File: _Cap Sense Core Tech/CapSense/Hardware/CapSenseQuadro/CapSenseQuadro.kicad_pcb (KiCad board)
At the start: 2 copper layers, 30 x 51.3 mm, 48 parts, among them IC1 FDC2214-rescue_FDC2214QRGHRQ1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, IC2 FDC2214QRGHRQ1, J1 Conn_02x04_Odd_Even, J2 Conn_02x04_Odd_Even, J3 Conn_02x01, SW1 SW_Push_DPDT, Y1 ECS-2033-400-BN

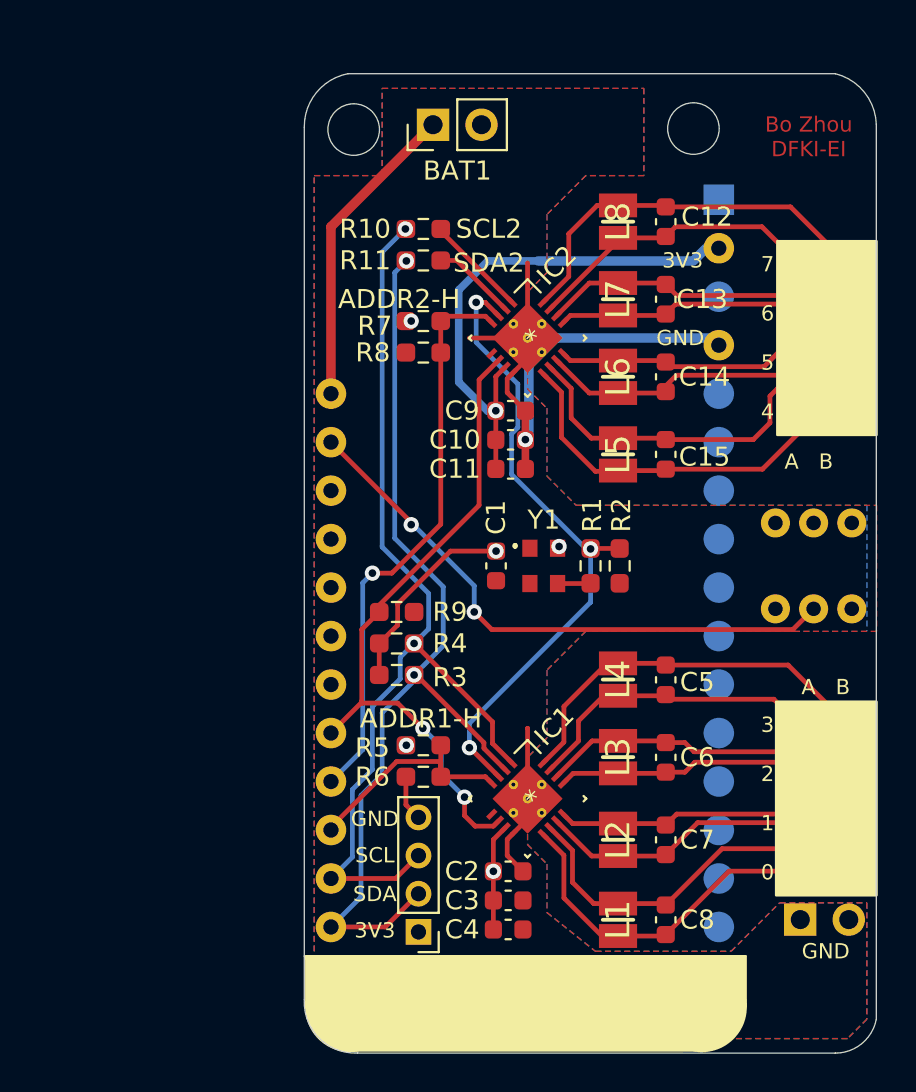
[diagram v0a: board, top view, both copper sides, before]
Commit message: pcb
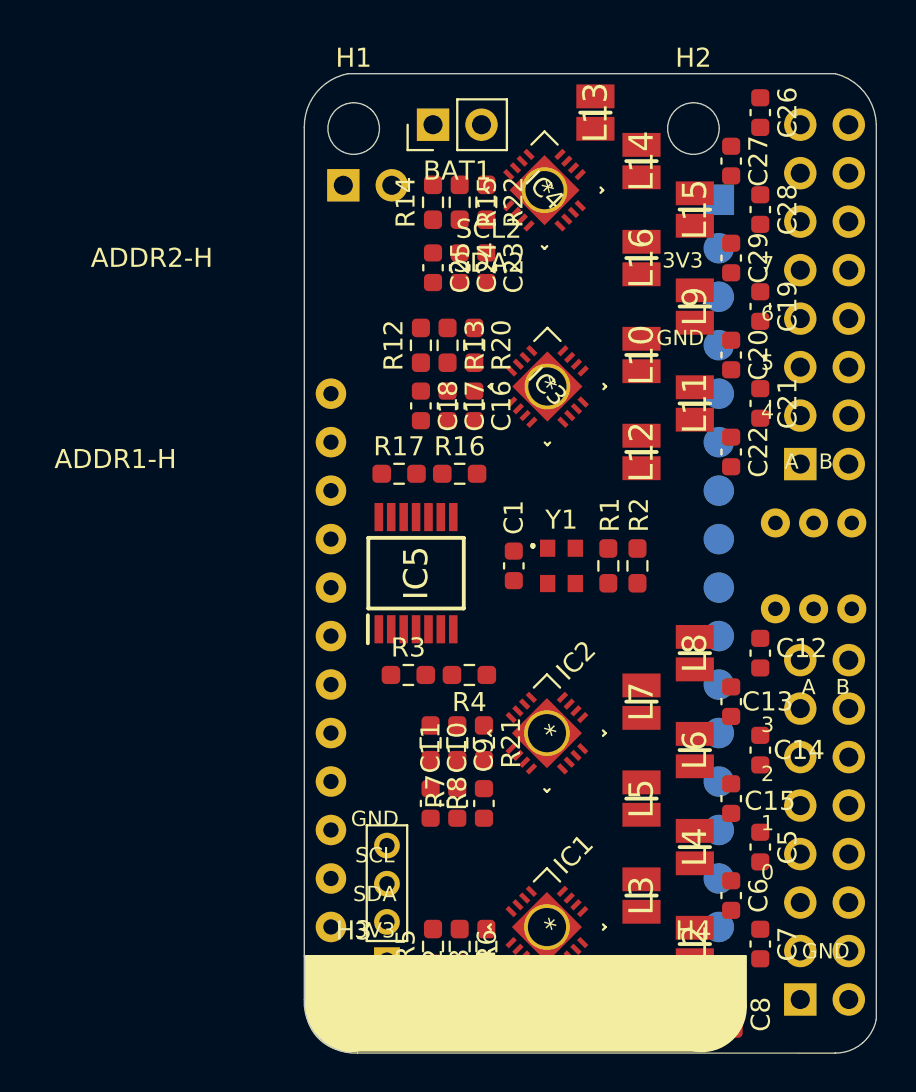
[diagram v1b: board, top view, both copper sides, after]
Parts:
- removed R10, R11: R, Resistor_SMD:R_0603_1608Metric_Pad0.98x0.95mm_HandSolder
- added C16: C, Capacitor_SMD:C_0603_1608Metric, F.Cu at (109.0, 117.2)
- added C17: C, Capacitor_SMD:C_0603_1608Metric, F.Cu at (107.6, 117.2)
- added C18: C, Capacitor_SMD:C_0603_1608Metric, F.Cu at (106.2, 117.2)
- added C19: Device_C, Capacitor_SMD:C_0603_1608Metric, F.Cu at (124.0, 112.0)
- added C20: Device_C, Capacitor_SMD:C_0603_1608Metric, F.Cu at (122.4, 114.6)
- added C21: Device_C, Capacitor_SMD:C_0603_1608Metric, F.Cu at (124.0, 117.1)
- added C22: Device_C, Capacitor_SMD:C_0603_1608Metric, F.Cu at (122.4, 119.6)
- added C23: C, Capacitor_SMD:C_0603_1608Metric, F.Cu at (109.6, 110.0)
- added C24: C, Capacitor_SMD:C_0603_1608Metric, F.Cu at (108.2, 110.0)
- added C25: C, Capacitor_SMD:C_0603_1608Metric, F.Cu at (106.8, 110.0)
- added C26: Device_C, Capacitor_SMD:C_0603_1608Metric, F.Cu at (124.0, 101.9)
- added C27: Device_C, Capacitor_SMD:C_0603_1608Metric, F.Cu at (122.4, 104.4)
- added C28: Device_C, Capacitor_SMD:C_0603_1608Metric, F.Cu at (124.0, 106.9)
- added C29: Device_C, Capacitor_SMD:C_0603_1608Metric, F.Cu at (122.4, 109.5)
- added IC3: FDC2214QRGHRQ1, FDC2214:FDC2214RGHR, F.Cu at (112.8, 116.2)
- added IC4: FDC2214QRGHRQ1, FDC2214:FDC2214RGHR, F.Cu at (112.6, 105.9)
- added IC5: PCA9543APWR, SamacSys:SOP65P640X120-14N, F.Cu at (105.9, 126.0)
- added L10: L0806C470MPWST, SamacSys:INDC2018X180N, F.Cu at (117.7, 114.6)
- added L11: L0806C470MPWST, SamacSys:INDC2018X180N, F.Cu at (120.5, 117.1)
- added L12: L0806C470MPWST, SamacSys:INDC2018X180N, F.Cu at (117.7, 119.6)
- added L13: L0806C470MPWST, SamacSys:INDC2018X180N, F.Cu at (115.3, 101.9)
- added L14: L0806C470MPWST, SamacSys:INDC2018X180N, F.Cu at (117.7, 104.4)
- added L15: L0806C470MPWST, SamacSys:INDC2018X180N, F.Cu at (120.5, 106.9)
- added L16: L0806C470MPWST, SamacSys:INDC2018X180N, F.Cu at (117.7, 109.5)
- added L9: L0806C470MPWST, SamacSys:INDC2018X180N, F.Cu at (120.5, 112.0)
- added R12: R, Resistor_SMD:R_0603_1608Metric_Pad0.98x0.95mm_HandSolder, F.Cu at (106.2, 114.0)
- added R13: R, Resistor_SMD:R_0603_1608Metric_Pad0.98x0.95mm_HandSolder, F.Cu at (107.6, 114.0)
- added R14: R, Resistor_SMD:R_0603_1608Metric_Pad0.98x0.95mm_HandSolder, F.Cu at (106.8, 106.6)
- added R15: R, Resistor_SMD:R_0603_1608Metric_Pad0.98x0.95mm_HandSolder, F.Cu at (108.2, 106.6)
- added R16: R, Resistor_SMD:R_0603_1608Metric_Pad0.98x0.95mm_HandSolder, F.Cu at (108.2, 120.8)
- added R17: R, Resistor_SMD:R_0603_1608Metric_Pad0.98x0.95mm_HandSolder, F.Cu at (105.0, 120.8)
- added R20: R, Resistor_SMD:R_0603_1608Metric_Pad0.98x0.95mm_HandSolder, F.Cu at (109.0, 114.0)
- added R21: R, Resistor_SMD:R_0603_1608Metric_Pad0.98x0.95mm_HandSolder, F.Cu at (109.5, 134.9)
- added R22: R, Resistor_SMD:R_0603_1608Metric_Pad0.98x0.95mm_HandSolder, F.Cu at (109.6, 106.6)
- J1, J2: value Conn_02x04_Odd_Even -> Conn_02x08_Odd_Even; footprint Connector_PinHeader_2.54mm:PinHeader_2x04_P2.54mm_Horizontal -> Connector_PinHeader_2.54mm:PinHeader_2x08_P2.54mm_Horizontal
- moved J3 45.3 mm to (102.1, 105.7)
- moved C12 23.1 mm to (124.0, 130.2)
- moved L8 23.0 mm to (120.5, 130.2)
- moved R7 22.1 mm to (106.7, 134.9), turned to 90 degrees
- moved C13 21.4 mm to (122.4, 132.7)
- moved L7 21.1 mm to (117.7, 132.7)
- moved IC2 20.7 mm to (112.8, 134.4)
- moved C9 20.6 mm to (109.5, 138.0), turned to -90 degrees
- moved R8 20.5 mm to (108.1, 134.9), turned to -90 degrees
- moved C14 20.2 mm to (124.0, 135.3)
- moved L6 20.0 mm to (120.5, 135.3)
- moved C10 19.3 mm to (108.1, 138.0), turned to -90 degrees
- moved C15 18.4 mm to (122.4, 137.8)
- moved R9 18.1 mm to (109.6, 145.5), turned to -90 degrees
- moved L5 18.1 mm to (117.7, 137.8)
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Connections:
- A1 pad 19: ADDR1 -> PCA0
- A1 pad 20: ADDR2 -> PCA1
- A1 pad 21: SD -> unconnected-(A1-Pad21)
- IC1 pad 1: SCL -> SCL0
- IC1 pad 2: SDA -> SDA0
- IC1 pad 6: SD -> SD1
- IC1 pad V: GND -> (no net)
- IC2 pad 1: SCL2 -> SCL0
- IC2 pad 2: SDA2 -> SDA0
- IC2 pad 6: SD -> SD2
- IC2 pad V: GND -> (no net)
- J2 pad 1: IN4A -> IN8A
- J2 pad 2: IN4B -> IN8B
- J2 pad 3: IN5A -> IN9A
- J2 pad 4: IN5B -> IN9B
- J2 pad 5: IN6A -> IN10A
- J2 pad 6: IN6B -> IN10B
- J2 pad 7: IN7A -> IN11A
- J2 pad 8: IN7B -> IN11B
- R3 pad 2: SDA -> SDA0
- R4 pad 2: SCL -> SCL0
- R9 pad 1: SD -> SD1
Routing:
- net SCL: track 51.1 -> 0.00 mm, vias 2 -> 0
- net SDA: track 50.9 -> 0.00 mm, vias 2 -> 0
- net +3V3: track 43.5 -> 0.00 mm, vias 6 -> 0
- net GND: track 37.4 -> 0.00 mm, vias 1 -> 0
- net SD: track 34.6 -> 0.00 mm, vias 2 -> 0
- net clk: track 33.7 -> 0.00 mm, vias 3 -> 0
- net Net-(A1-Pad27): track 30.7 -> 0.00 mm, vias 2 -> 0
- net ADDR2: track 30.0 -> 0.00 mm, vias 1 -> 0
- net IN7B: track 20.7 -> 0.00 mm
- net IN3B: track 20.6 -> 0.00 mm
- net IN4B: track 20.6 -> 0.00 mm
- net IN0B: track 20.0 -> 0.00 mm
- net IN4A: track 18.9 -> 0.00 mm
- net IN0A: track 18.4 -> 0.00 mm
- net IN6B: track 16.9 -> 0.00 mm
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- removed copper zone on B.Cu, net +3V3
- removed copper zone on F.Cu, net GND
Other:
- board text removed: "Bo Zhou DFKI-EI"
